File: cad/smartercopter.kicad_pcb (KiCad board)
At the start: 2 copper layers, 37.7 x 16.8 mm, 74 parts, among them P1 CONN_5, P2 CONN_01X01, P3 CONN_01X01, P4 CONN_2, P5 CONN_01X01, P6 CONN_01X01, P7 CONN_01X01, Q1 SiA910EDJ, SW1 SW_PUSH_4, U1 CC2541, U2 MPU-9250, U3 TPS73001, U4 TPS73001, U5 DRV8837, X1 32Mhz

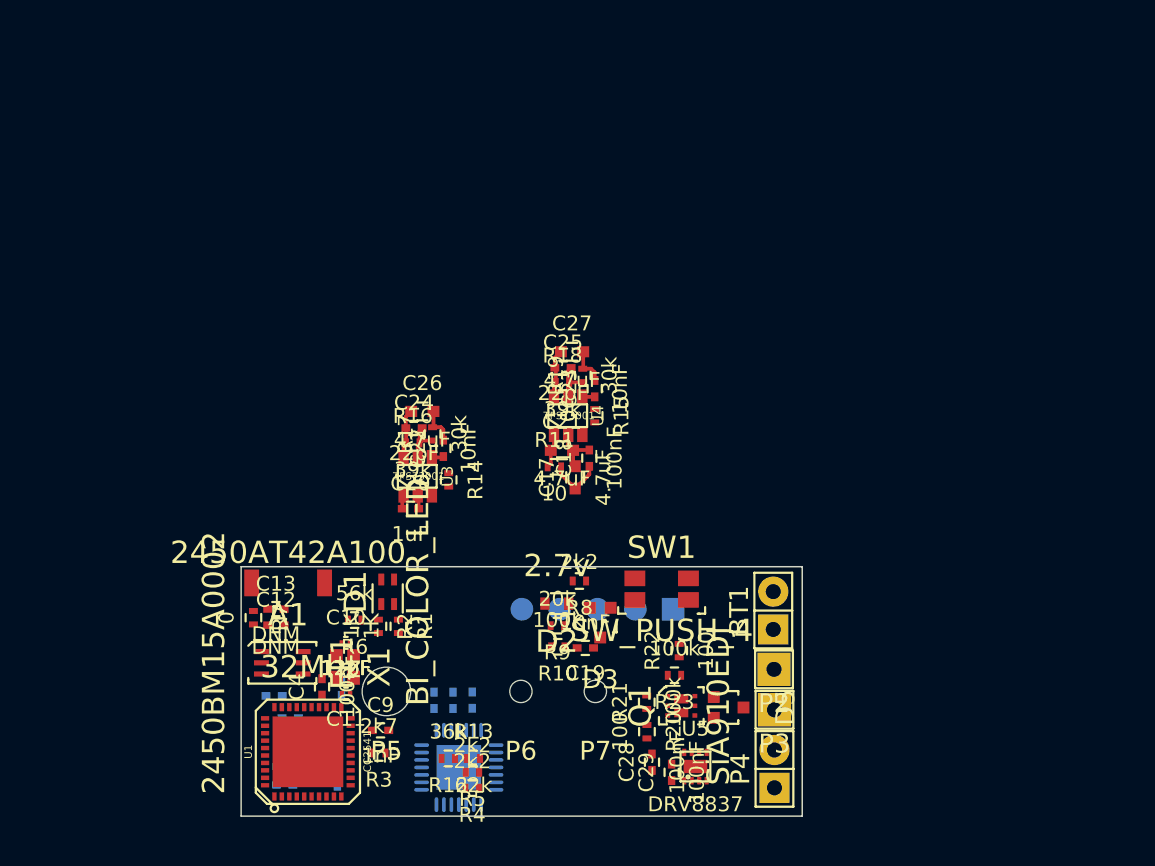
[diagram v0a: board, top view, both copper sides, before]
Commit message: routed some stuff
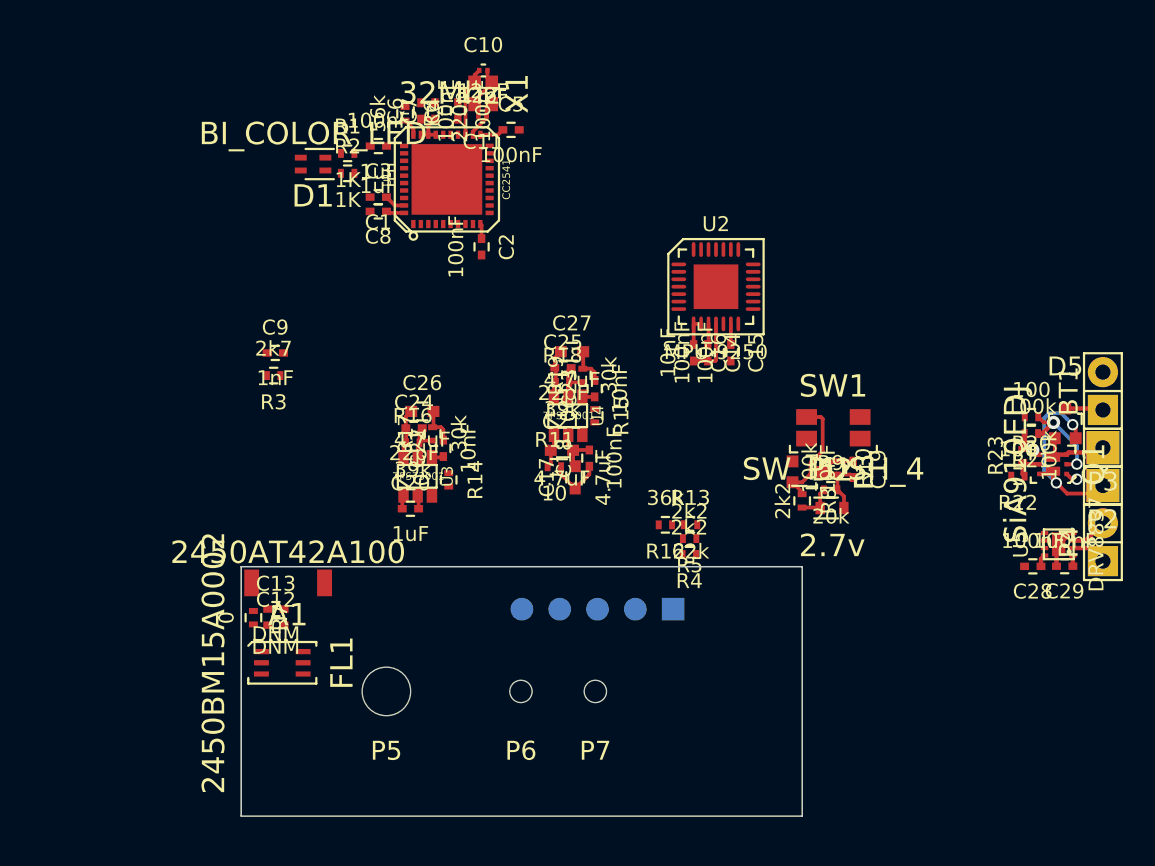
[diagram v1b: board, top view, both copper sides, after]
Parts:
- C1, C14, C15, C16, C2, C3, C5, C6, C7, C8, U2: moved to F.Cu
- moved C6 41.7 mm to (63.4, 73.9), turned to 90 degrees
- moved C7 40.8 mm to (64.3, 73.9), turned to 90 degrees
- moved C3 40.1 mm to (60.5, 76.2), turned to 180 degrees
- moved C11 39.8 mm to (67.5, 74.3)
- moved C4 39.8 mm to (65.9, 73.9)
- moved X1 39.6 mm to (67.6, 72.7)
- moved U1 39.6 mm to (65.1, 78.5)
- moved C10 39.6 mm to (67.6, 71.2)
- moved C5 39.1 mm to (69.5, 75.2), turned to 0 degrees
- moved C8 39.0 mm to (60.5, 80.6), turned to 180 degrees
- moved C1 38.8 mm to (60.5, 79.7), turned to 180 degrees
- moved C2 37.0 mm to (67.5, 83.0), turned to 270 degrees
- moved U2 36.6 mm to (83.2, 85.7)
- moved R6 34.2 mm to (62.3, 74.1), turned to 270 degrees
- moved R20 33.4 mm to (104.4, 94.4), turned to 180 degrees
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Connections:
- P2 pad 1: Net-(D5-Pad1) -> Net-(D5-Pad2)
- P3 pad 1: Net-(D5-Pad2) -> Net-(D5-Pad1)
- Q1 pad 3: Net-(D5-Pad2) -> Net-(D5-Pad1)
- Q1 pad 6: Net-(D5-Pad1) -> Net-(D5-Pad2)
- Q1 pad D1: Net-(D5-Pad1) -> Net-(D5-Pad2)
- Q1 pad D2: Net-(D5-Pad2) -> Net-(D5-Pad1)
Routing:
- net Net-(D5-Pad2): track 0.00 -> 15.5 mm, vias 0 -> 2
- net GND: track 4.35 -> 14.6 mm, vias 0 -> 2
- net VCCA: track 3.28 -> 11.4 mm
- net Net-(D3-Pad2): track 0.00 -> 7.69 mm
- net Net-(Q1-Pad2): track 0.00 -> 6.68 mm, vias 0 -> 2
- net Net-(D5-Pad1): track 0.00 -> 5.58 mm
- net /XOSC_Q2: track 0.00 -> 4.70 mm
- net AGND: track 2.60 -> 6.56 mm
- net DGND: track 2.58 -> 6.38 mm
- net VCC: track 3.32 -> 6.58 mm
- net +BATT: track 4.68 -> 7.93 mm
- net /XOSC_Q1: track 0.00 -> 2.58 mm
- net /power/BUTTON: track 0.00 -> 2.55 mm
- net Net-(P4-Pad2): track 0.00 -> 2.50 mm
- net Net-(P4-Pad1): track 0.00 -> 2.38 mm
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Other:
- net class Default: clearance 0.254 -> 0.0508; via_dia 0.889 -> 0.762; via_drill 0.635 -> 0.508
- rule trace_clearance: 0.254 -> 0.0508
- rule via_min_size: 0.889 -> 0.762

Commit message: stuff on board with a bit of routing
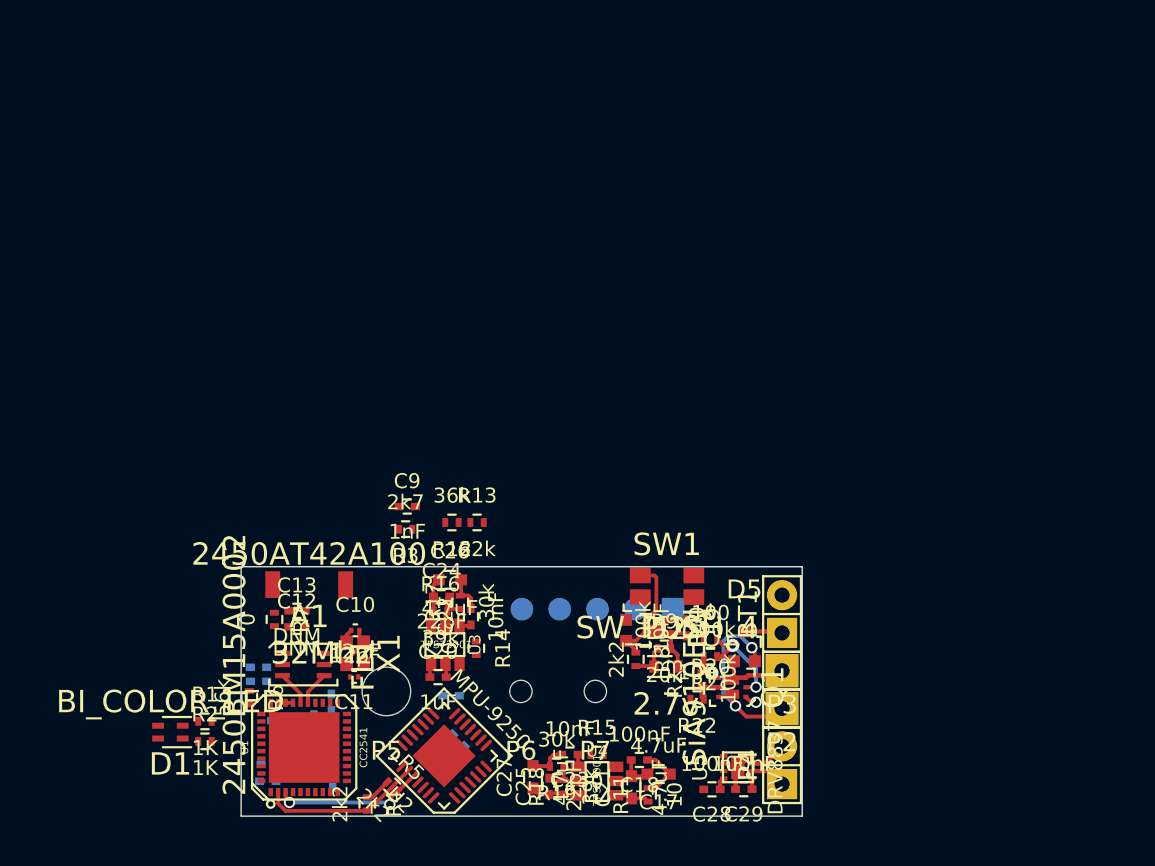
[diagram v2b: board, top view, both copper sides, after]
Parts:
- C1, C14, C15, C16, C2, C3, C4, C5, C6, C7, C8: moved to B.Cu
- moved C4 42.2 mm to (56.2, 115.0), turned to 270 degrees
- moved R6 40.6 mm to (51.9, 113.3)
- moved C5 40.3 mm to (57.4, 113.6), turned to 270 degrees
- moved C6 39.8 mm to (52.5, 112.2), turned to 180 degrees
- moved D1 39.4 mm to (46.6, 115.6)
- moved R1 39.4 mm to (48.9, 114.9)
- moved R2 39.4 mm to (48.9, 116.2)
- moved U1 39.4 mm to (55.6, 116.7)
- moved C7 39.2 mm to (52.5, 111.3), turned to 180 degrees
- moved C3 39.2 mm to (53.9, 114.9), turned to 0 degrees
- moved C8 39.0 mm to (53.1, 118.9), turned to 0 degrees
- moved C1 38.8 mm to (53.2, 117.8), turned to 0 degrees
- moved C11 38.6 mm to (58.9, 111.9)
- moved C10 38.6 mm to (59.0, 108.8)
- moved X1 38.6 mm to (59.0, 110.3)
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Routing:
- net /sensors/SCL: track 0.00 -> 10.7 mm
- net /sensors/SDA: track 0.00 -> 10.1 mm, vias 0 -> 2
- net VCCA: track 11.4 -> 6.07 mm
- net AGND: track 6.56 -> 2.60 mm
- net /XOSC_Q2: track 4.70 -> 0.94 mm
- net /XOSC_Q1: track 2.58 -> 0.00 mm
- net VCC: track 6.58 -> 4.15 mm
- net /RF_N: track 0.00 -> 2.32 mm
- net /RF_P: track 0.00 -> 2.28 mm
- net Net-(C14-Pad1): track 1.41 -> 0.18 mm
- net Net-(C8-Pad1): track 1.23 -> 0.00 mm
- net Net-(R6-Pad2): track 1.19 -> 0.00 mm
- net DGND: track 6.38 -> 5.79 mm

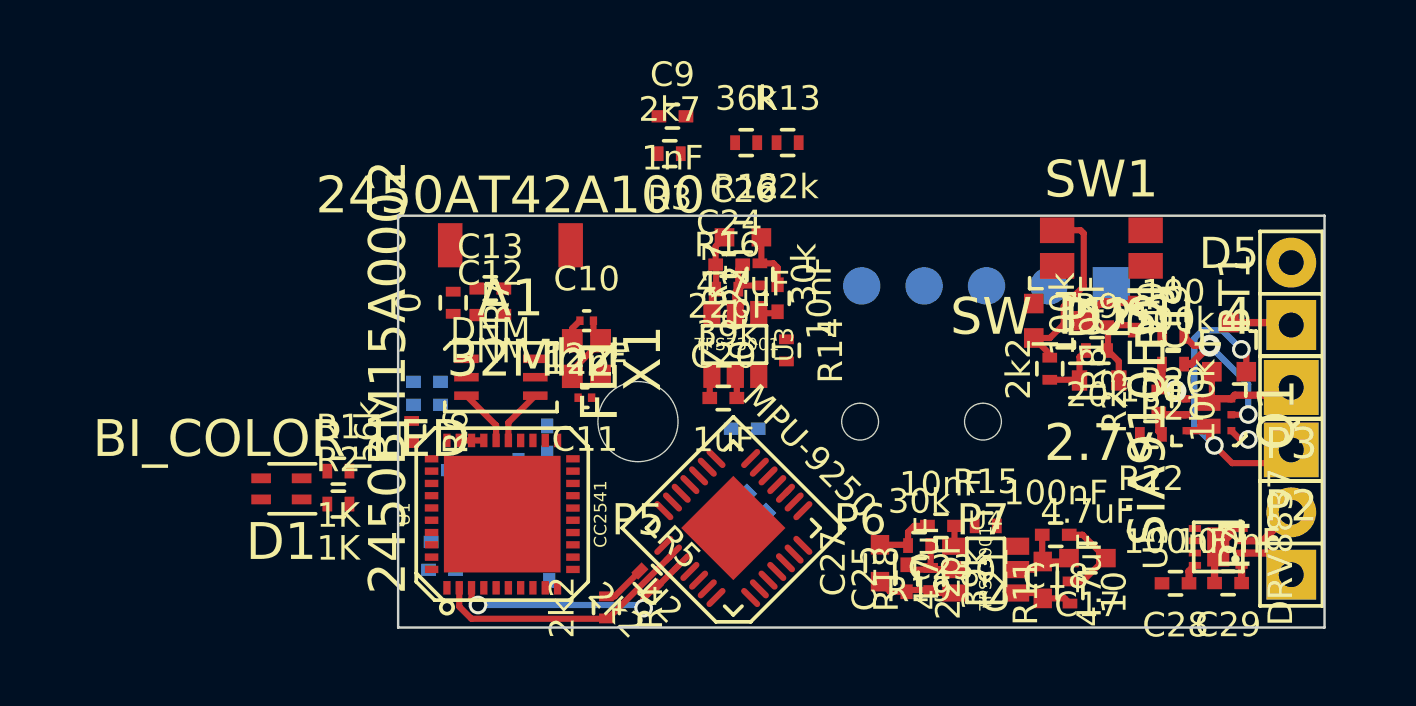
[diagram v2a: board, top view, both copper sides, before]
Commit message: stuff on board
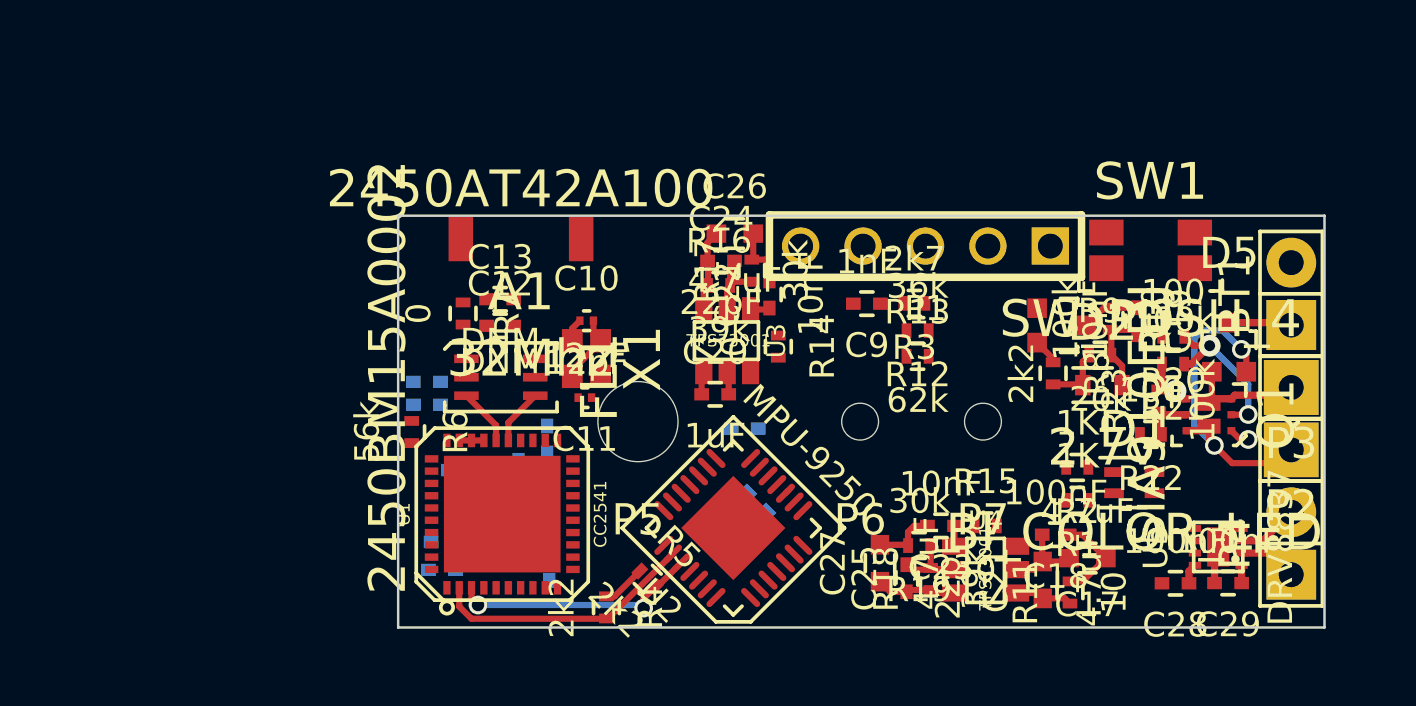
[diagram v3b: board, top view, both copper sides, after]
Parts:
- P1: moved to F.Cu
- moved D1 34.7 mm to (81.3, 115.4), turned to 180 degrees
- moved R2 30.1 mm to (79.0, 114.8), turned to 180 degrees
- moved R1 30.1 mm to (79.0, 116.1), turned to 180 degrees
- moved R3 11.7 mm to (72.3, 108.1)
- moved C9 11.0 mm to (70.4, 108.1), turned to 180 degrees
- moved R12 10.4 mm to (72.5, 109.2)
- moved R13 10.2 mm to (72.5, 110.2)
- moved P1 2.97 mm to (72.8, 105.8)
- moved SW1 2.01 mm to (81.9, 105.9)
- moved C12 0.59 mm to (55.5, 109.0)
- moved C13 0.59 mm to (55.5, 107.9)
- moved R7 0.59 mm to (54.0, 108.5)
- moved A1 0.50 mm to (56.3, 105.5)
- moved C20 0.36 mm to (64.2, 111.8)
- moved C22 0.36 mm to (66.4, 107.7)
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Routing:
- net Net-(D3-Pad2): track 7.69 -> 1.07 mm

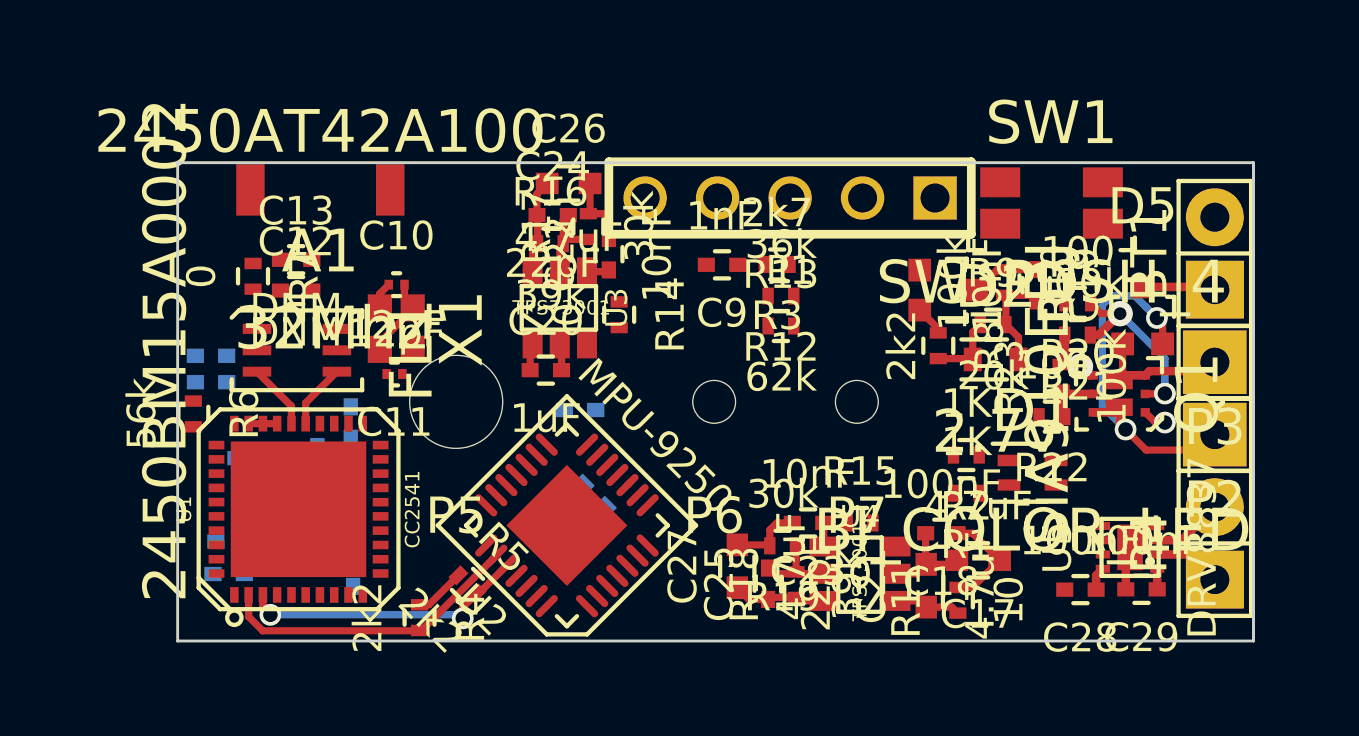
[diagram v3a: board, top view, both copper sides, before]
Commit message: progress check in
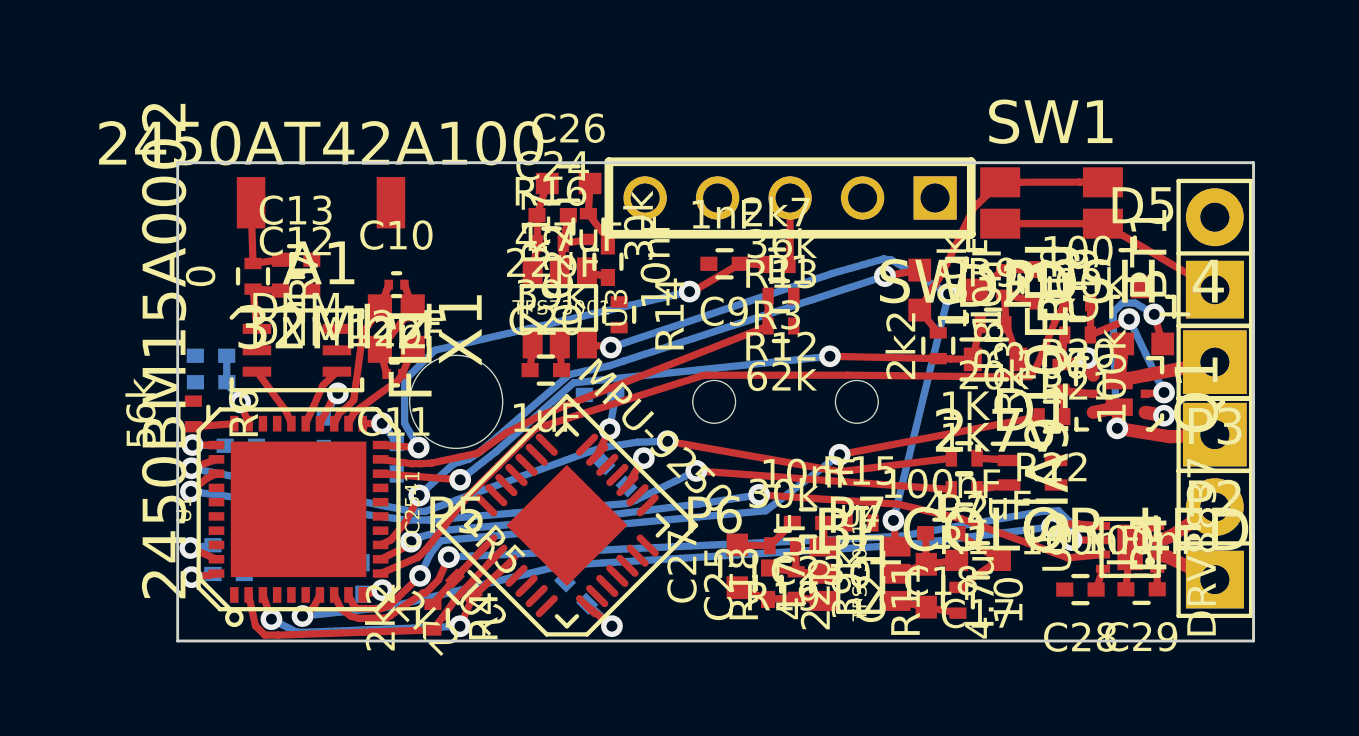
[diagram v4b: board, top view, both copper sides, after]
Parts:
- moved C16 2.44 mm to (65.3, 119.6)
- moved C5 2.04 mm to (59.0, 114.9)
- moved C4 1.07 mm to (56.4, 114.0)
- moved C14 1.02 mm to (66.7, 115.5)
- moved C15 0.88 mm to (66.1, 112.7), turned to 180 degrees
- moved C3 0.58 mm to (53.5, 114.4)
- moved R4 0.47 mm to (60.3, 120.4)
- moved A1 0.45 mm to (56.3, 105.9)
- moved C2 0.43 mm to (57.8, 119.1)
- moved C22 0.27 mm to (66.4, 108.0)
- moved C1 0.17 mm to (53.1, 117.9)
- moved R5 0.16 mm to (61.3, 119.4)
- moved R1 0.15 mm to (78.9, 116.0)
- moved R2 0.13 mm to (78.9, 114.9)
- moved C9 0.09 mm to (70.5, 108.1)
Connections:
- C19 pad 1: Net-(C19-Pad1) -> /power/EN_REG
- D3 pad 3: Net-(C19-Pad1) -> /power/EN_REG
- R10 pad 1: Net-(C19-Pad1) -> /power/EN_REG
- U1 pad 32: /LED1 -> /LED2
- U1 pad 33: /LED2 -> /LED1
- U3 pad 3: /power/EN -> /power/EN_REG
- U4 pad 3: /power/EN -> /power/EN_REG
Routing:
- net /motor/EN: track 0.00 -> 29.3 mm, vias 0 -> 2
- net /motor/PH: track 0.00 -> 29.1 mm, vias 0 -> 2
- net /LED2: track 0.00 -> 28.2 mm, vias 0 -> 2
- net /LED1: track 0.00 -> 28.1 mm, vias 0 -> 2
- net /motor/UP_ROTOR: track 0.00 -> 28.0 mm
- net /motor/LOW_ROTOR: track 0.00 -> 26.5 mm, vias 0 -> 2
- net /motor/nSLEEP: track 0.00 -> 26.0 mm, vias 0 -> 2
- net /power/EN_REG: track 0.00 -> 25.9 mm, vias 0 -> 3
- net /power/EN: track 0.00 -> 21.9 mm, vias 0 -> 2
- net /power/BUTTON: track 2.55 -> 23.3 mm, vias 0 -> 2
- net Net-(C9-Pad1): track 0.00 -> 17.4 mm, vias 0 -> 2
- net /power/BATTVOLT: track 0.00 -> 15.6 mm
- net VCCA: track 6.07 -> 18.7 mm, vias 0 -> 6
- net Net-(D3-Pad2): track 1.07 -> 9.98 mm
- net +BATT: track 7.93 -> 13.3 mm
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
